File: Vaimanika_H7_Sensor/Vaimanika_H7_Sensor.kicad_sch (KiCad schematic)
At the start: 71 parts, among them SW1 TS-1088-AR02016, U1 TCAN334G, U2 STM32H743VITx, U3 NCP163ASN330T1G, U4 MS5611-01BA, U5 ICM-42688-P, U6 ICM-42688-P, U7 W25Q128JVS, U8 RT9080-33GJ5, U9 BMI088, Y1 25 MHz

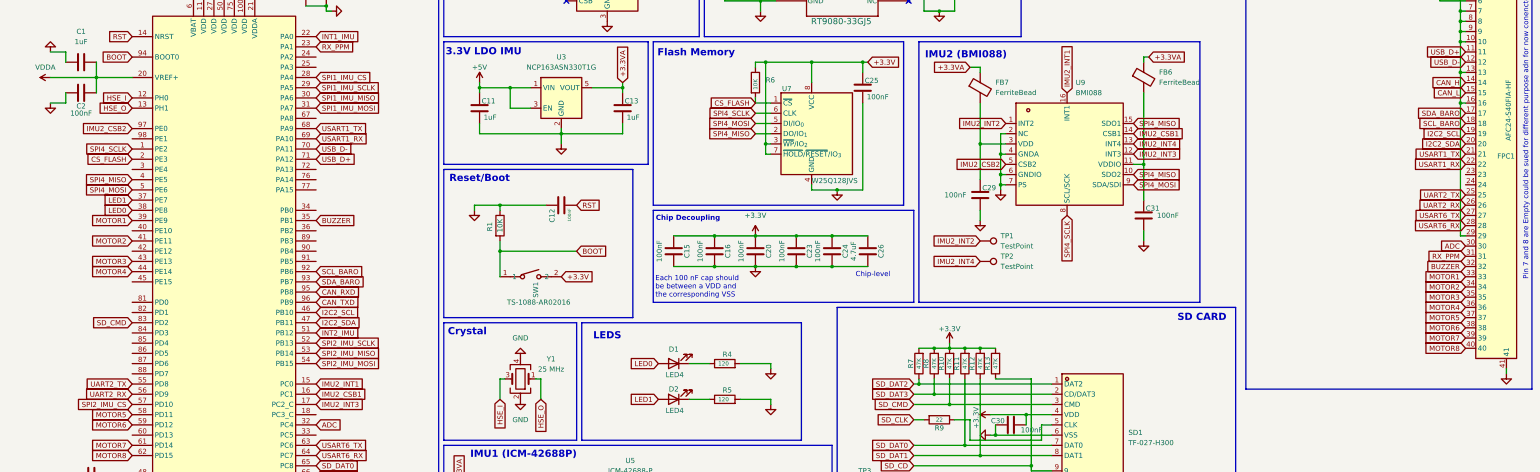
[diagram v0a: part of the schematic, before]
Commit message: 01-05-2026
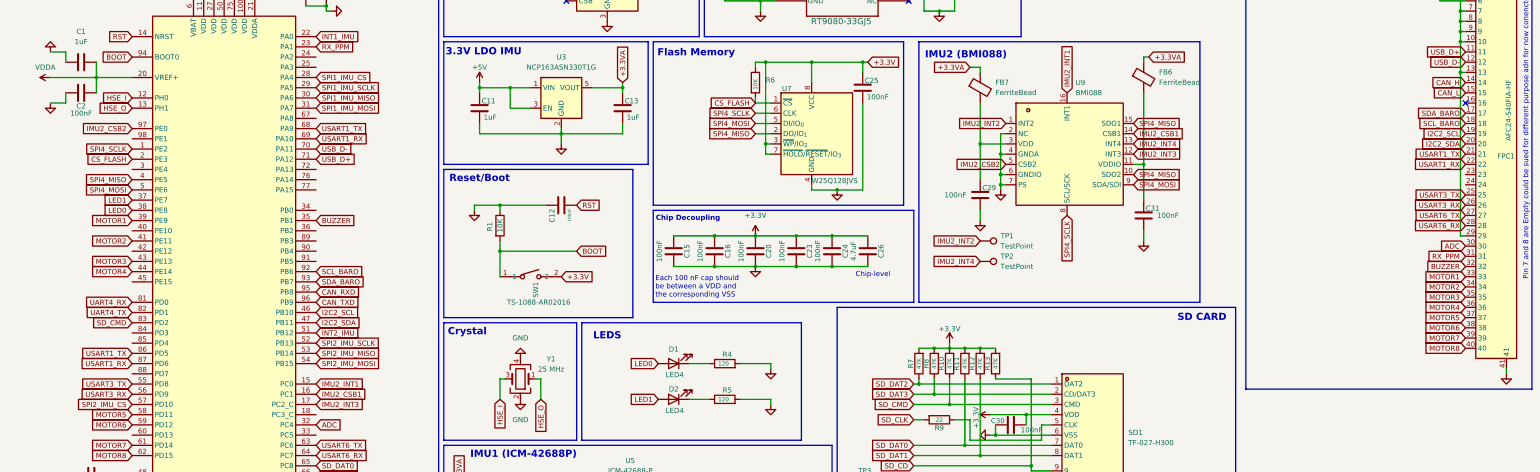
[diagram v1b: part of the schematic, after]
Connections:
- net GND: no longer FPC1.16
- net USART1_RX: now also U2.87 (PD6)
- net USART1_TX: now also U2.86 (PD5)
- net UART4_RX: now reaches U2.81 (PD0)
- net UART4_TX: now reaches U2.82 (PD1)
- net UART2_RX renamed USART3_RX
- net UART2_TX renamed USART3_TX
- no-connect marks 9 -> 10
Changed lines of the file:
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@@
 	)
 	(junction
-		(at 388.62 67.31)
-		(diameter 0)
-		(color 0 0 0 0)
-	)
-	(junction
 		(at 388.62 59.69)
 		(diameter 0)
@@
 	)
 	(no_connect
+		(at 389.89 67.31)
+	)
+	(no_connect
 		(at 158.75 213.36)
 	)
@@
 	(wire
 		(pts
-			(xy 389.89 67.31) (xy 388.62 67.31)
-		)
-		(stroke
-			(width 0)
-			(type default)
-		)
-	)
-	(wire
-		(pts
 			(xy 388.62 46.99) (xy 388.62 44.45)
 		)
@@
 	(wire
 		(pts
-			(xy 388.62 59.69) (xy 388.62 67.31)
+			(xy 388.62 59.69) (xy 388.62 100.33)
 		)
 		(stroke
@@
 	(wire
 		(pts
-			(xy 388.62 67.31) (xy 388.62 100.33)
-		)
-		(stroke
-			(width 0)
-			(type default)
-		)
-	)
-	(wire
-		(pts
 			(xy 144.78 72.39) (xy 144.78 74.93)
 		)
@@
 		)
 	)
-	(global_label "UART2_TX"
+	(global_label "USART3_TX"
 		(shape input)
 		(at 389.89 90.17 180)
@@
 		)
 		(property "Intersheetrefs" "${INTERSHEET_REFS}"
-			(at 377.8939 90.17 0)
+			(at 376.6844 90.17 0)
 			(effects
 				(font
@@
 		)
 	)
+	(global_label "UART4_TX"
+		(shape input)
+		(at 58.42 119.38 180)
+		(fields_autoplaced yes)
+		(effects
+			(font
+				(size 1.27 1.27)
+			)
+			(justify right)
+		)
+		(property "Intersheetrefs" "${INTERSHEET_REFS}"
+			(at 46.4239 119.38 0)
+			(effects
+				(font
+					(size 1.27 1.27)
+					(italic yes)
+				)
+				(justify right)
+				(hide yes)
+			)
+		)
+	)
 	(global_label "MOTOR8"
 		(shape input)
@@
 		)
 	)
+	(global_label "USART1_RX"
+		(shape input)
+		(at 58.42 132.08 180)
+		(fields_autoplaced yes)
+		(effects
+			(font
+				(size 1.27 1.27)
+			)
+			(justify right)
+		)
+		(property "Intersheetrefs" "${INTERSHEET_REFS}"
+			(at 44.912 132.08 0)
+			(effects
+				(font
+					(size 1.27 1.27)
+					(italic yes)
+				)
+				(justify right)
+				(hide yes)
+			)
+		)
+	)
 	(global_label "BUZZER"
 		(shape input)
@@
 		)
 	)
-	(global_label "UART2_RX"
+	(global_label "USART3_RX"
 		(shape input)
 		(at 58.42 139.7 180)
@@
 		)
 		(property "Intersheetrefs" "${INTERSHEET_REFS}"
-			(at 46.1215 139.7 0)
+			(at 44.912 139.7 0)
 			(effects
 				(font
@@
 		)
 	)
-	(global_label "UART2_TX"
+	(global_label "USART3_TX"
 		(shape input)
 		(at 58.42 137.16 180)
@@
 		)
 		(property "Intersheetrefs" "${INTERSHEET_REFS}"
-			(at 46.4239 137.16 0)
+			(at 45.2144 137.16 0)
 			(effects
 				(font
@@
 		)
 	)
-	(global_label "UART2_RX"
+	(global_label "USART3_RX"
 		(shape input)
 		(at 389.89 92.71 180)
@@
 		)
 		(property "Intersheetrefs" "${INTERSHEET_REFS}"
-			(at 377.5915 92.71 0)
+			(at 376.382 92.71 0)
 			(effects
 				(font
@@
 		)
 	)
+	(global_label "UART4_RX"
+		(shape input)
+		(at 58.42 116.84 180)
+		(fields_autoplaced yes)
+		(effects
+			(font
+				(size 1.27 1.27)
+			)
+			(justify right)
+		)
+		(property "Intersheetrefs" "${INTERSHEET_REFS}"
+			(at 46.1215 116.84 0)
+			(effects
+				(font
+					(size 1.27 1.27)
+					(italic yes)
+				)
+				(justify right)
+				(hide yes)
+			)
+		)
+	)
 	(global_label "SPI2_IMU_MISO"
 		(shape input)
@@
 			(effects
 				(font
+					(size 1.27 1.27)
+					(italic yes)
+				)
+				(justify right)
+				(hide yes)
+			)
+		)
+	)
+	(global_label "USART1_TX"
+		(shape input)
+		(at 58.42 129.54 180)
+		(fields_autoplaced yes)
+		(effects
+			(font
+				(size 1.27 1.27)
+			)
+			(justify right)
+		)
+		(property "Intersheetrefs" "${INTERSHEET_REFS}"
+			(at 45.2144 129.54 0)
+			(effects
+				(font

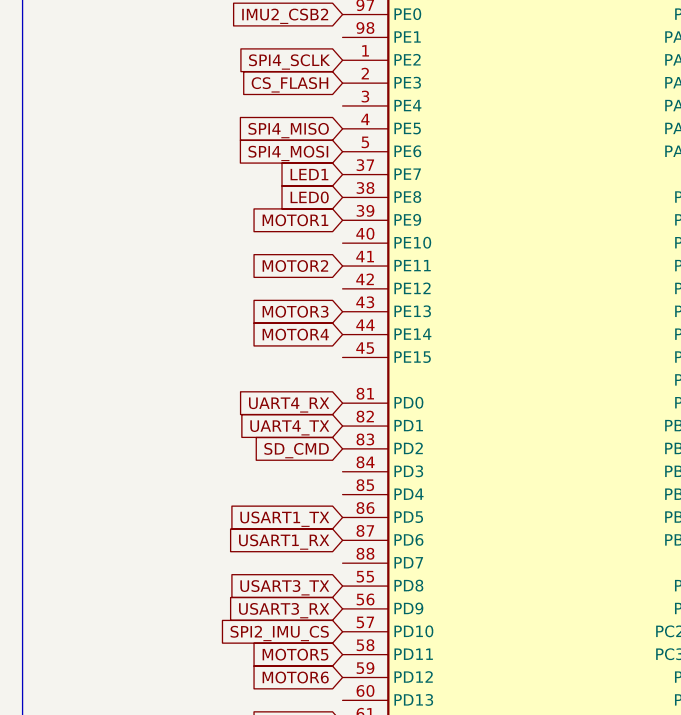
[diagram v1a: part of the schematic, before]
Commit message: 18-05-2026
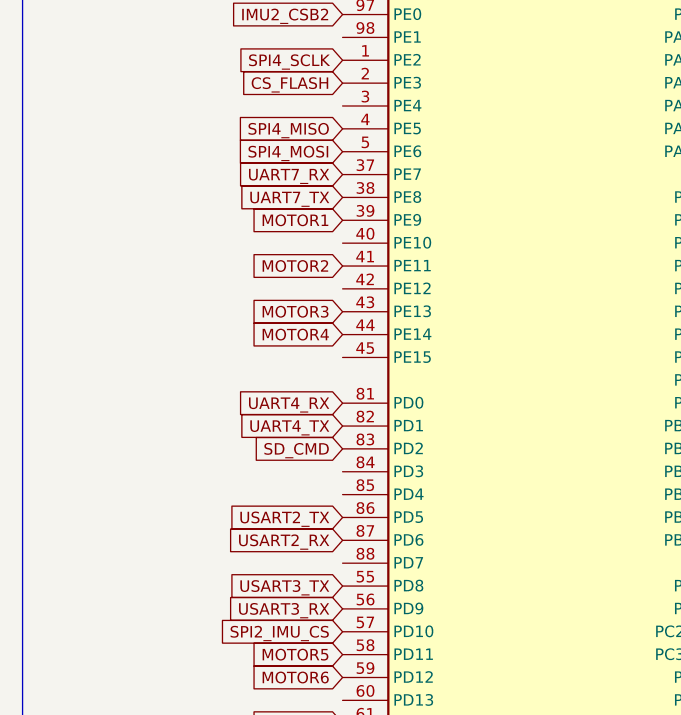
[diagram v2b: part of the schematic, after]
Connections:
- net LED0: no longer U2.38 (PE8)
- net LED1: no longer U2.37 (PE7)
- net USART1_RX: no longer U2.87 (PD6)
- net USART1_TX: no longer U2.86 (PD5)
- new net UART7_RX: U2.37 (PE7)
- new net UART7_TX: U2.38 (PE8)
- new net USART2_RX: U2.87 (PD6)
- new net USART2_TX: U2.86 (PD5)
